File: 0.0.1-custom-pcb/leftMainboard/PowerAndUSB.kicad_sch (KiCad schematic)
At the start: 31 parts, among them J1 USB-C USB2 receptacle (footpr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, J2 53398-0371, Q2 P-channel MOSFET (guess), Q3 P-channel MOSFET (guess), SW1 TK-6580A-1, U1 SY7088DGC, U2 TP4056-42-ESOP8, U3 PRTR5V0U2X

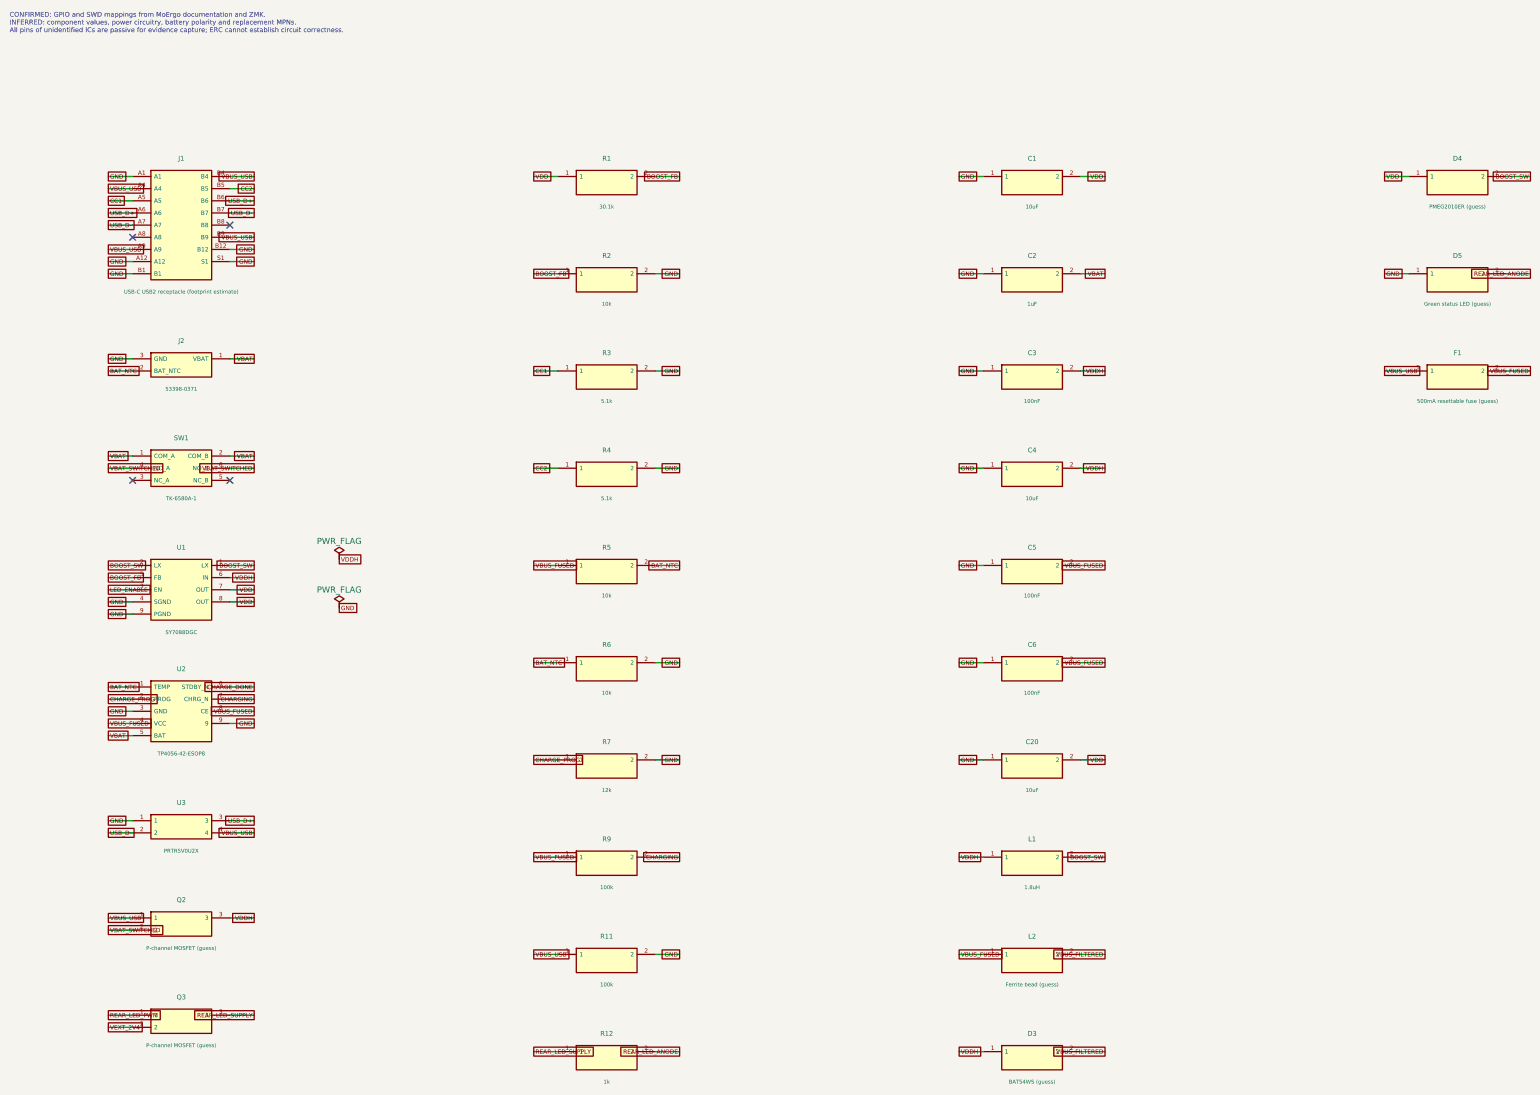
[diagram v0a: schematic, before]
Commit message: update more of left main
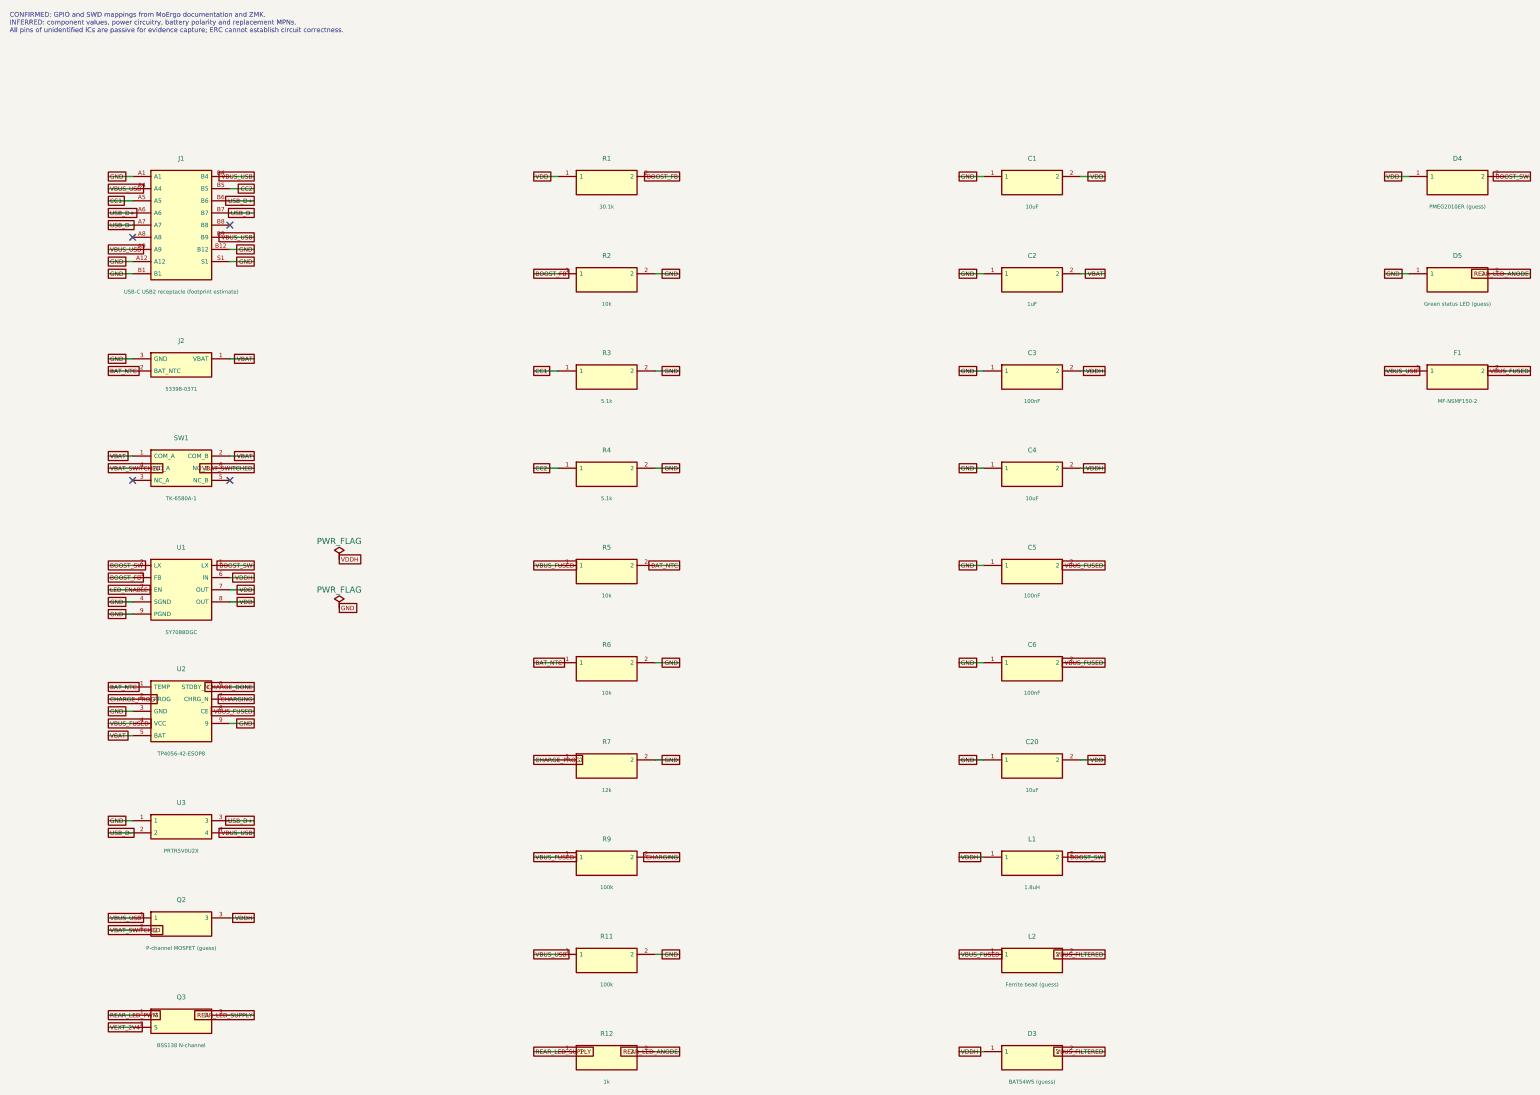
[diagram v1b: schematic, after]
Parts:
- F1: value 500mA resettable fuse (guess) -> MF-NSMF150-2; Confidence Medium (function), Low (rating) -> User selected; Evidence Gold B-marked rectangular part is likely PPTC USB protection -> Selected by user from the 8 marking and measured 3.4 x 1.8 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; LCSC (none) -> C89655; LCSC Part (none) -> C89655; MPN (none) -> MF-NSMF150-2; Manufacturer (none) -> Bourns
- Q3: value P-channel MOSFET (guess) -> BSS138 N-channel; Candidate part AO3401A / SI2301 family -> BSS138; Confidence Low -> Medium; Evidence 3-lead packages; faint SS/G marking; polarity and part numb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 -> User measured body about 3x1.3 mm, marking SS; diode-mode d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; LCSC (none) -> C7420339
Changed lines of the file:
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@@
 (property "Reference" "Q3" (at 55.88 218.47999999999996 0)
 (effects (font (size 1.0 1.0))))
-(property "Value" "P-channel MOSFET (guess)" (at 55.88 228.55999999999995 0)
+(property "Value" "BSS138 N-channel" (at 55.88 228.55999999999995 0)
 (effects (font (size 0.8 0.8))))
 (property "Footprint" "Reconstruction:Q3_SOT-23" (at 55.88 223.51999999999995 0)
 (effects (font (size 1.0 1.0))
 (hide yes)))
-(property "Datasheet" "" (at 55.88 223.51999999999995 0)
-(effects (font (size 1.0 1.0))
-(hide yes)))
-(property "Confidence" "Low" (at 55.88 223.51999999999995 0)
-(effects (font (size 1.0 1.0))
-(hide yes)))
-(property "Evidence" "3-lead packages; faint SS/G marking; polarity and part number unconfirmed" (at 55.88 223.51999999999995 0)
-(effects (font (size 1.0 1.0))
-(hide yes)))
-(property "Candidate part" "AO3401A / SI2301 family" (at 55.88 223.51999999999995 0)
+(property "Datasheet" "https://www.lcsc.com/datasheet/C7420339.pdf" (at 55.88 223.51999999999995 0)
+(effects (font (size 1.0 1.0))
+(hide yes)))
+(property "LCSC" "C7420339" (at 55.88 223.51999999999995 0)
+(effects (font (size 1.0 1.0))
+(hide yes)))
+(property "Confidence" "Medium" (at 55.88 223.51999999999995 0)
+(effects (font (size 1.0 1.0))
+(hide yes)))
+(property "Evidence" "User measured body about 3x1.3 mm, marking SS; diode-mode display 440 (about 0.440 V), pins 1/2 shorted, red 2 black 3; supports N-channel; reverse reading and isolated-device test not reported; exact MPN unconfirmed" (at 55.88 223.51999999999995 0)
+(effects (font (size 1.0 1.0))
+(hide yes)))
+(property "Candidate part" "BSS138" (at 55.88 223.51999999999995 0)
 (effects (font (size 1.0 1.0))
 (hide yes)))
@@
 (property "Reference" "F1" (at 322.58000000000004 83.85999999999999 0)
 (effects (font (size 1.0 1.0))))
-(property "Value" "500mA resettable fuse (guess)" (at 322.58000000000004 93.94 0)
+(property "Value" "MF-NSMF150-2" (at 322.58000000000004 93.94 0)
 (effects (font (size 0.8 0.8))))
 (property "Footprint" "Reconstruction:F1_Fuse_1206_3216Metric" (at 322.58000000000004 88.89999999999999 0)
 (effects (font (size 1.0 1.0))
 (hide yes)))
-(property "Datasheet" "" (at 322.58000000000004 88.89999999999999 0)
-(effects (font (size 1.0 1.0))
-(hide yes)))
-(property "Confidence" "Medium (function), Low (rating)" (at 322.58000000000004 88.89999999999999 0)
-(effects (font (size 1.0 1.0))
-(hide yes)))
-(property "Evidence" "Gold B-marked rectangular part is likely PPTC USB protection" (at 322.58000000000004 88.89999999999999 0)
-(effects (font (size 1.0 1.0))
-(hide yes)))
-(property "Candidate part" "" (at 322.58000000000004 88.89999999999999 0)
+(property "Datasheet" "https://www.bourns.com/docs/product-datasheets/mf-nsmf.pdf" (at 322.58000000000004 88.89999999999999 0)
+(effects (font (size 1.0 1.0))
+(hide yes)))
+(property "Confidence" "User selected" (at 322.58000000000004 88.89999999999999 0)
+(effects (font (size 1.0 1.0))
+(hide yes)))
+(property "Evidence" "Selected by user from the 8 marking and measured 3.4 x 1.8 mm package" (at 322.58000000000004 88.89999999999999 0)
+(effects (font (size 1.0 1.0))
+(hide yes)))
+(property "MPN" "MF-NSMF150-2" (at 322.58000000000004 88.89999999999999 0)
 (effects (font (size 1.0 1.0))
 (hide yes)))
@@
 (pin "2")
 (instances (project "leftMainboard" (path "/eac6e0a1-0901-4c4d-b0b4-c941afc6d33b/3d4a4145-dfbf-4d53-839d-da2f670b524e" (reference "F1")
-(unit 1)))))
+(unit 1))))
+(property "Description" "Bourns MF-NSMF150-2 resettable PPTC fuse; 1.5A hold, 3A trip, 6V; 1206 package; marking 8" (at 0 0 0) (effects (font (size 1 1)) (hide yes)))
+(property "Manufacturer" "Bourns" (at 0 0 0) (effects (font (size 1 1)) (hide yes)))
+(property "LCSC" "C89655" (at 0 0 0) (effects (font (size 1 1)) (hide yes)))
+(property "LCSC Part" "C89655" (at 0 0 0) (effects (font (size 1 1)) (hide yes)))
+)
 (text "CONFIRMED: GPIO and SWD mappings from MoErgo documentation and ZMK.\nINFERRED: component values, power circuitry, battery polarity and replacement MPNs.\nAll pins of unidentified ICs are passive for evidence capture; ERC cannot establish circuit correctness." (at 20 15 0)
 (effects (font (size 1.0 1.0))
